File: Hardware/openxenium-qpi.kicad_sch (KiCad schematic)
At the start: 34 parts, among them J1 SPI/LED, J2 UART, Q1 NPN, Q2 NPN, Q3 NPN, Q4 NPN, Q5 NPN, U1 XC3S50A-VQG100, U2 W25Q128JVSIQ, U3 W25Q128JVSIQ, U4 W25Q128JVSIQ, U5 NCV8164ASN120T1G

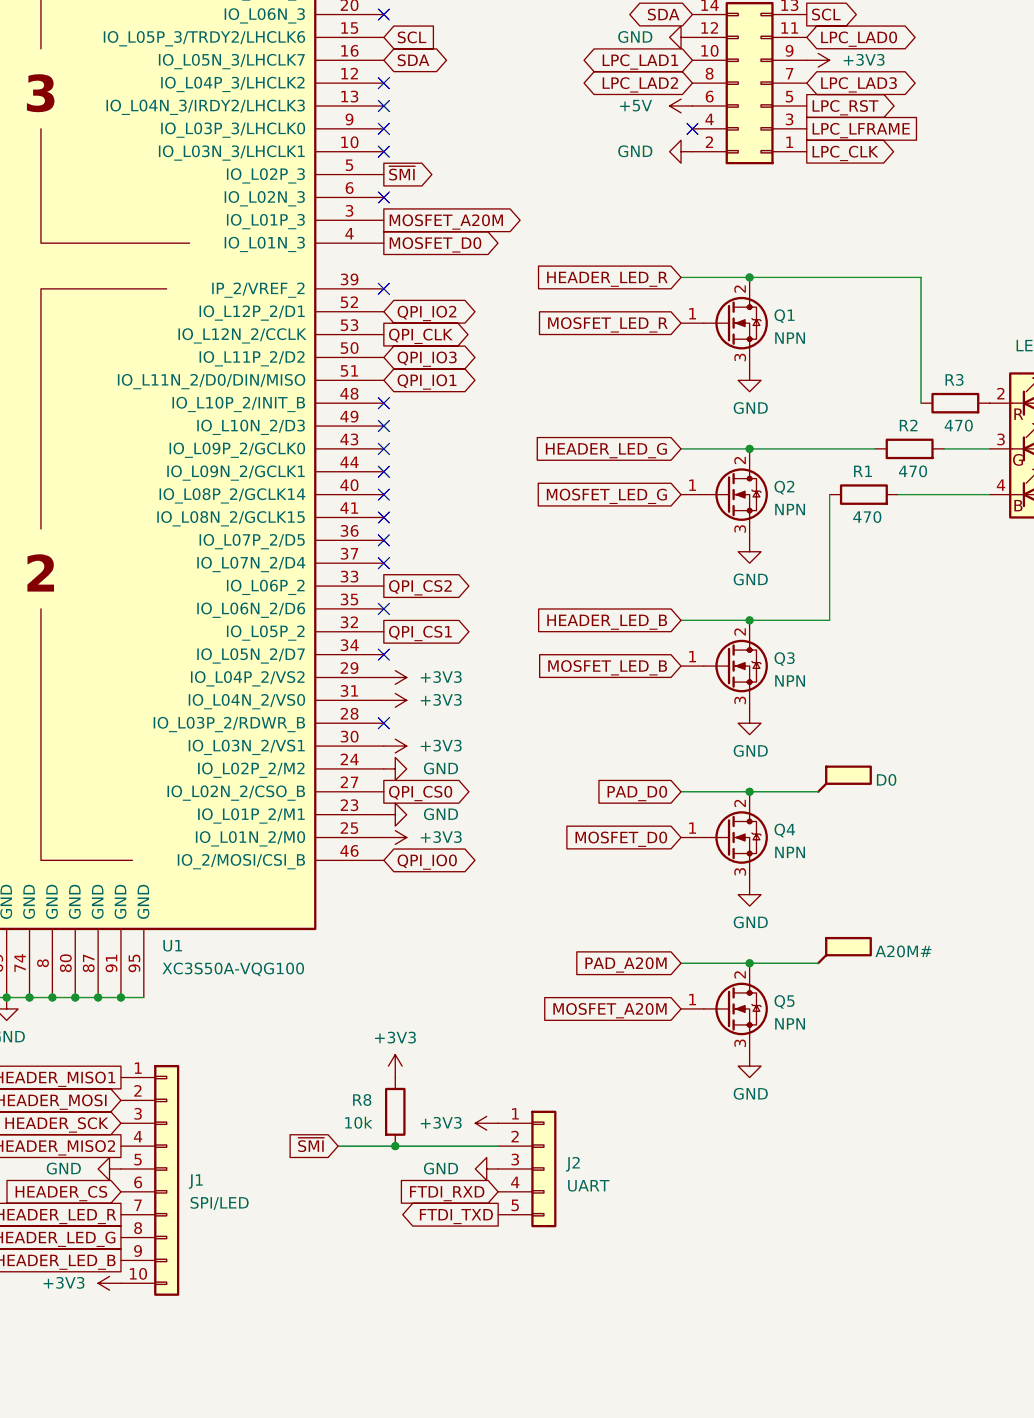
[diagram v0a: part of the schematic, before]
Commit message: HW: Import Rev. 20230304 QPI board
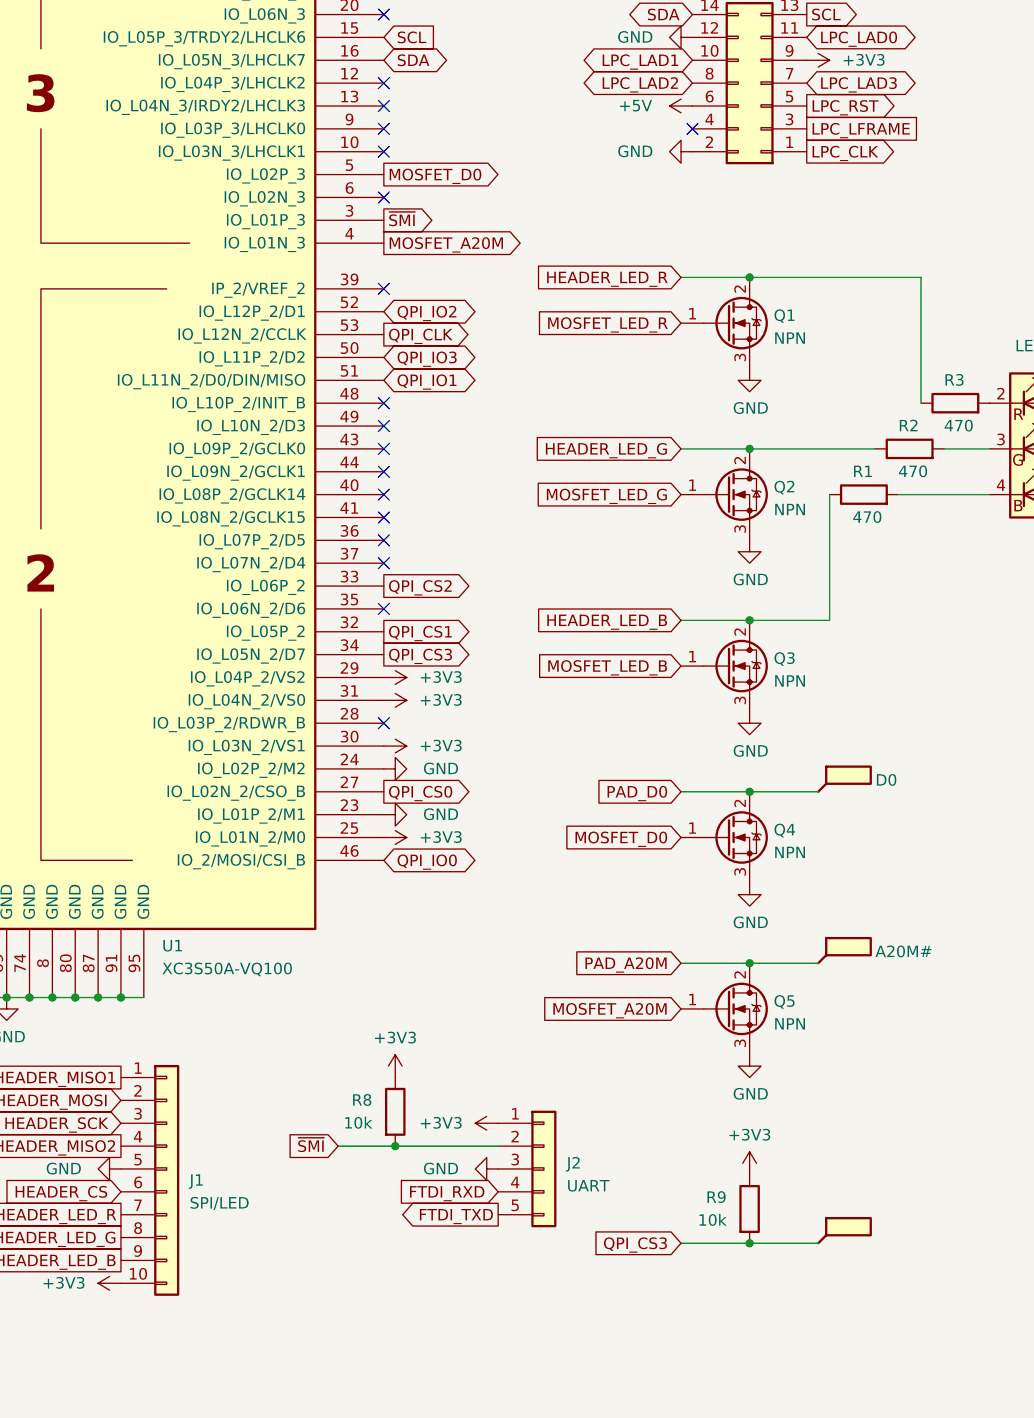
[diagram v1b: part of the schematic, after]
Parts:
- added R9: 10k, symbol Device:R
- added TP?: (no value), symbol Connector:TestPoint_Flag
- U1: value XC3S50A-VQG100 -> XC3S50A-VQ100; symbol FPGA_Xilinx:XC3S50A-VQG100 -> FPGA_Xilinx:XC3S50A-VQ100
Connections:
- net +3V3: now also R9.1
- net MOSFET_A20M: now also U1.4 (IO_L01N_3); no longer U1.3 (IO_L01P_3)
- net MOSFET_D0: now also U1.5 (IO_L02P_3); no longer U1.4 (IO_L01N_3)
- net ~{SMI}: now also U1.3 (IO_L01P_3); no longer U1.5 (IO_L02P_3)
- net QPI_CS3: now reaches U1.34 (IO_L05N_2/D7)
- net QPI_CS3: now also R9.2, TP?.1
- no-connect marks 32 -> 31
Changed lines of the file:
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@@
   (title_block
     (title "Original Xbox OpenXenium QPI")
-    (date "2022-07-04")
-    (rev "20220704")
+    (date "2023-03-04")
+    (rev "20230304")
     (company "XboxDev")
     (comment 2 "Licensed under CERN OHL v.1.2 or later")
@@
   )
   (junction (at 66.04 199.39) (diameter 0) (color 0 0 0 0)
+  )
+  (junction (at 156.21 226.695) (diameter 0) (color 0 0 0 0)
   )
   (junction (at 179.07 71.12) (diameter 0) (color 0 0 0 0)
@@
   (no_connect (at 115.57 151.13))
   (no_connect (at 115.57 156.21))
-  (no_connect (at 115.57 161.29))
   (no_connect (at 115.57 140.97))
   (no_connect (at 115.57 138.43))
@@
     (stroke (width 0) (type default) (color 0 0 0 0))
   )
+  (wire (pts (xy 148.59 226.695) (xy 156.21 226.695))
+    (stroke (width 0) (type default) (color 0 0 0 0))
+  )
   (wire (pts (xy 156.21 119.38) (xy 175.26 119.38))
     (stroke (width 0) (type default) (color 0 0 0 0))
@@
   )
   (wire (pts (xy 85.09 26.67) (xy 99.06 26.67))
+    (stroke (width 0) (type default) (color 0 0 0 0))
+  )
+  (wire (pts (xy 156.21 226.695) (xy 163.83 226.695))
     (stroke (width 0) (type default) (color 0 0 0 0))
   )
@@
     )
   )
-  (global_label "MOSFET_A20M" (shape output) (at 115.57 113.03 0) (fields_autoplaced)
-    (effects (font (size 1.27 1.27)) (justify left))
-    (property "Intersheet References" "${INTERSHEET_REFS}" (id 0) (at 131.1064 112.9506 0)
+  (global_label "MOSFET_A20M" (shape output) (at 115.57 115.57 0) (fields_autoplaced)
+    (effects (font (size 1.27 1.27)) (justify left))
+    (property "Intersheet References" "${INTERSHEET_REFS}" (id 0) (at 131.1064 115.4906 0)
       (effects (font (size 1.27 1.27)) (justify left) hide)
     )
@@
     )
   )
+  (global_label "QPI_CS3" (shape output) (at 115.57 161.29 0) (fields_autoplaced)
+    (effects (font (size 1.27 1.27)) (justify left))
+    (property "Intersheet References" "${INTERSHEET_REFS}" (id 0) (at 125.7561 161.2106 0)
+      (effects (font (size 1.27 1.27)) (justify left) hide)
+    )
+  )
   (global_label "HEADER_MOSI" (shape output) (at 31.75 116.84 180) (fields_autoplaced)
     (effects (font (size 1.27 1.27)) (justify right))
@@
     )
   )
+  (global_label "QPI_CS3" (shape input) (at 148.59 226.695 180) (fields_autoplaced)
+    (effects (font (size 1.27 1.27)) (justify right))
+    (property "Intersheet References" "${INTERSHEET_REFS}" (id 0) (at 138.4039 226.6156 0)
+      (effects (font (size 1.27 1.27)) (justify right) hide)
+    )
+  )
   (global_label "QPI_IO2" (shape bidirectional) (at 115.57 123.19 0) (fields_autoplaced)
     (effects (font (size 1.27 1.27)) (justify left))
@@
     )
   )
-  (global_label "~{SMI}" (shape output) (at 115.57 107.95 0) (fields_autoplaced)
-    (effects (font (size 1.27 1.27)) (justify left))
-    (property "Intersheet References" "${INTERSHEET_REFS}" (id 0) (at 121.1599 107.8706 0)
+  (global_label "~{SMI}" (shape output) (at 115.57 113.03 0) (fields_autoplaced)
+    (effects (font (size 1.27 1.27)) (justify left))
+    (property "Intersheet References" "${INTERSHEET_REFS}" (id 0) (at 121.1599 112.9506 0)
       (effects (font (size 1.27 1.27)) (justify left) hide)
     )
@@
     )
   )
-  (global_label "MOSFET_D0" (shape output) (at 115.57 115.57 0) (fields_autoplaced)
-    (effects (font (size 1.27 1.27)) (justify left))
-    (property "Intersheet References" "${INTERSHEET_REFS}" (id 0) (at 128.6269 115.4906 0)
+  (global_label "MOSFET_D0" (shape output) (at 115.57 107.95 0) (fields_autoplaced)
+    (effects (font (size 1.27 1.27)) (justify left))
+    (property "Intersheet References" "${INTERSHEET_REFS}" (id 0) (at 128.6269 107.8706 0)
       (effects (font (size 1.27 1.27)) (justify left) hide)
     )
@@
     (pin "1")
   )
+  (symbol (lib_id "Connector:TestPoint_Flag") (at 163.83 226.695 0) (unit 1)
+    (in_bom yes) (on_board yes)
+    (property "Reference" "TP?" (id 0) (at 170.434 224.4633 0)
+      (effects (font (size 1.27 1.27)) (justify left) hide)
+    )
+    (property "Value" "" (id 1) (at 170.18 225.425 0)
+      (effects (font (size 1.27 1.27)) (justify left))
+    )
+    (property "Footprint" "" (id 2) (at 168.91 226.695 0)
+      (effects (font (size 1.27 1.27)) hide)
+    )
+    (property "Datasheet" "~" (id 3) (at 168.91 226.695 0)
+      (effects (font (size 1.27 1.27)) hide)
+    )
+    (pin "1")
+  )
   (symbol (lib_id "Device:Q_NMOS_GDS") (at 153.67 181.61 0) (unit 1)
     (in_bom yes) (on_board yes) (fields_autoplaced)
@@
     (pin "2")
   )
+  (symbol (lib_id "Device:R") (at 156.21 222.885 0) (unit 1)
+    (in_bom yes) (on_board yes)
+    (property "Reference" "R9" (id 0) (at 153.67 221.615 0)
+      (effects (font (size 1.27 1.27)) (justify right))
+    )
+    (property "Value" "10k" (id 1) (at 153.67 224.155 0)
+      (effects (font (size 1.27 1.27)) (justify right))
+    )
+    (property "Footprint" "" (id 2) (at 154.432 222.885 90)
+      (effects (font (size 1.27 1.27)) hide)
+    )
+    (property "Datasheet" "~" (id 3) (at 156.21 222.885 0)
+      (effects (font (size 1.27 1.27)) hide)
+    )
+    (pin "1")
+    (pin "2")
+  )
   (symbol (lib_id "power:GND") (at 115.57 179.07 90) (unit 1)
     (in_bom yes) (on_board yes)
@@
     )
     (property "Datasheet" "" (id 3) (at 135.89 63.5 0)
+      (effects (font (size 1.27 1.27)) hide)
+    )
+    (pin "1")
+  )
+  (symbol (lib_id "power:+3V3") (at 156.21 219.075 0) (unit 1)
+    (in_bom yes) (on_board yes)
+    (property "Reference" "#PWR?" (id 0) (at 156.21 222.885 0)
+      (effects (font (size 1.27 1.27)) hide)
+    )
+    (property "Value" "+3V3" (id 1) (at 156.21 214.6808 0))
+    (property "Footprint" "" (id 2) (at 156.21 219.075 0)
+      (effects (font (size 1.27 1.27)) hide)
+    )
+    (property "Datasheet" "" (id 3) (at 156.21 219.075 0)
       (effects (font (size 1.27 1.27)) hide)
     )
@@
     (pin "2")
   )
-  (symbol (lib_id "FPGA_Xilinx:XC3S50A-VQG100") (at 86.36 152.4 0) (unit 1)
+  (symbol (lib_id "FPGA_Xilinx:XC3S50A-VQ100") (at 86.36 152.4 0) (unit 1)
     (in_bom yes) (on_board yes) (fields_autoplaced)
     (property "Reference" "U1" (id 0) (at 90.9194 193.6734 0)
       (effects (font (size 1.27 1.27)) (justify left))
     )
-    (property "Value" "XC3S50A-VQG100" (id 1) (at 90.9194 196.2103 0)
+    (property "Value" "XC3S50A-VQ100" (id 1) (at 90.9194 196.2103 0)
       (effects (font (size 1.27 1.27)) (justify left))
     )
@@
       (reference "#PWR?") (unit 1) (value "+3V3") (footprint "")
     )
+    (path "/4c4d8c01-f08c-4001-924d-9e67fab08564"
+      (reference "#PWR?") (unit 1) (value "+3V3") (footprint "")
+    )
     (path "/5606e02e-672e-4a2d-889c-a111fbab5339"
       (reference "#PWR?") (unit 1) (value "+3V3") (footprint "")
@@
       (reference "R8") (unit 1) (value "10k") (footprint "")
     )
+    (path "/3e2119d5-6d7c-4c5e-9c0e-b1126a651835"
+      (reference "R9") (unit 1) (value "10k") (footprint "")
+    )
     (path "/dfdae403-bb08-48d4-b042-b5f0fa182e90"
       (reference "RN1") (unit 1) (value "10k") (footprint "")
     )
+    (path "/2147ed10-10d3-4476-ac4b-0f117afbd209"
+      (reference "TP?") (unit 1) (value "CS3") (footprint "")
+    )
     (path "/82d553b0-aca7-43ac-9320-93c9eb56322b"
       (reference "TP?") (unit 1) (value "D0") (footprint "")
@@
     )
     (path "/dd541050-73b9-4ab3-a94b-b1a82baf515d"
-      (reference "U1") (unit 1) (value "XC3S50A-VQG100") (footprint "")
+      (reference "U1") (unit 1) (value "XC3S{50,200}A-VQ100") (footprint "")
     )
     (path "/8c22bbfd-7175-4e8c-92a3-1b5ef1ebb6f4"
